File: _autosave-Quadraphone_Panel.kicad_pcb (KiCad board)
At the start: 2 copper layers, 60.8 x 128.5 mm, 30 parts

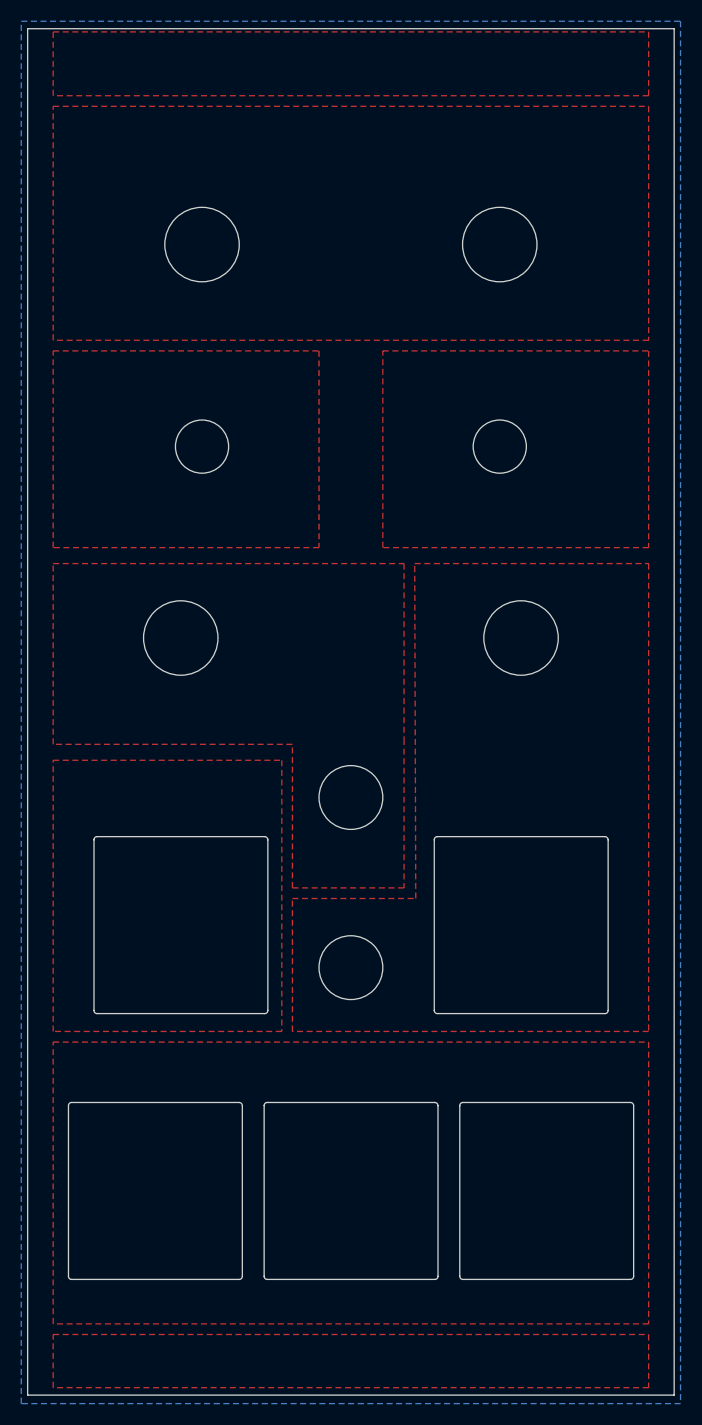
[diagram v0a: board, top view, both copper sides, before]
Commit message: Refinements to panel and controls
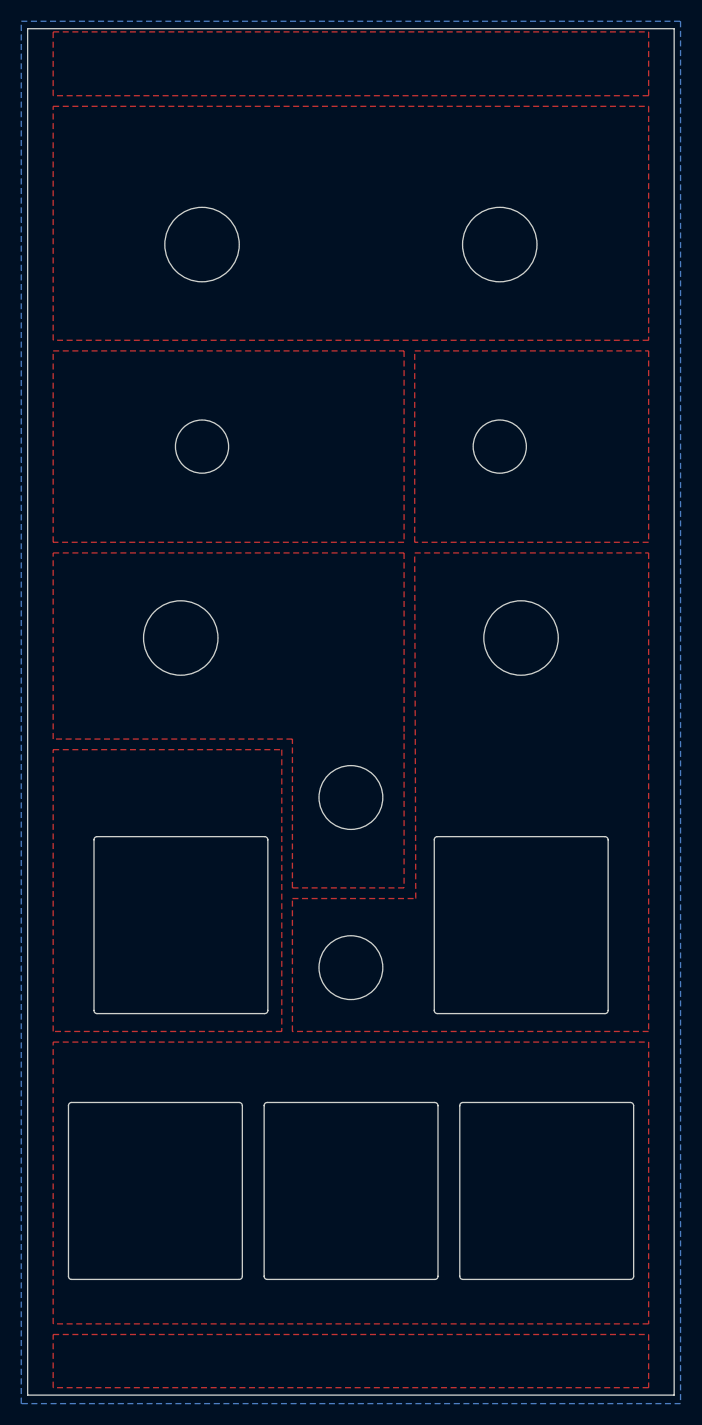
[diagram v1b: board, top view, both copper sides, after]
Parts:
- removed kibuzzard-63D1288B: G***, kibuzzard-63D1288B
- removed kibuzzard-63D1404C: G***, kibuzzard-63D1404C
- added kibuzzard-63D25E01: G***, kibuzzard-63D25E01, F.Cu at (90.0, 70.0)
- added kibuzzard-63D25EC7: G***, kibuzzard-63D25EC7, F.Cu at (80.0, 100.1)
- moved kibuzzard-63D139E5 5.52 mm to (64.0, 108.5)
- moved kibuzzard-63D1286A 1.00 mm to (90.0, 82.0)
